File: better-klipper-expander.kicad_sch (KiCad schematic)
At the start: 90 parts, among them J1 24V IN, J10 TH1, J11 VFAN_SEL1, J12 Neopixel, J13 VFAN_SEL2, J2 USB4105-GF-A, J3 FAN0, J4 FAN1, J5 FAN2, J6 TH0, J7 FAN3, J8 FAN4, J9 FAN5, Q1 AO3400C, Q2 AO3400C, Q3 AO3400C, Q4 AO3400C, Q5 AO3400C, Q6 AO3400C, U1 W25Q80DVSNIG, U2 XT1861B332MR-G, U3 TPS5450DDAR, U4 RP2040, U5 TXS0101DBVR, Y1 12MHz

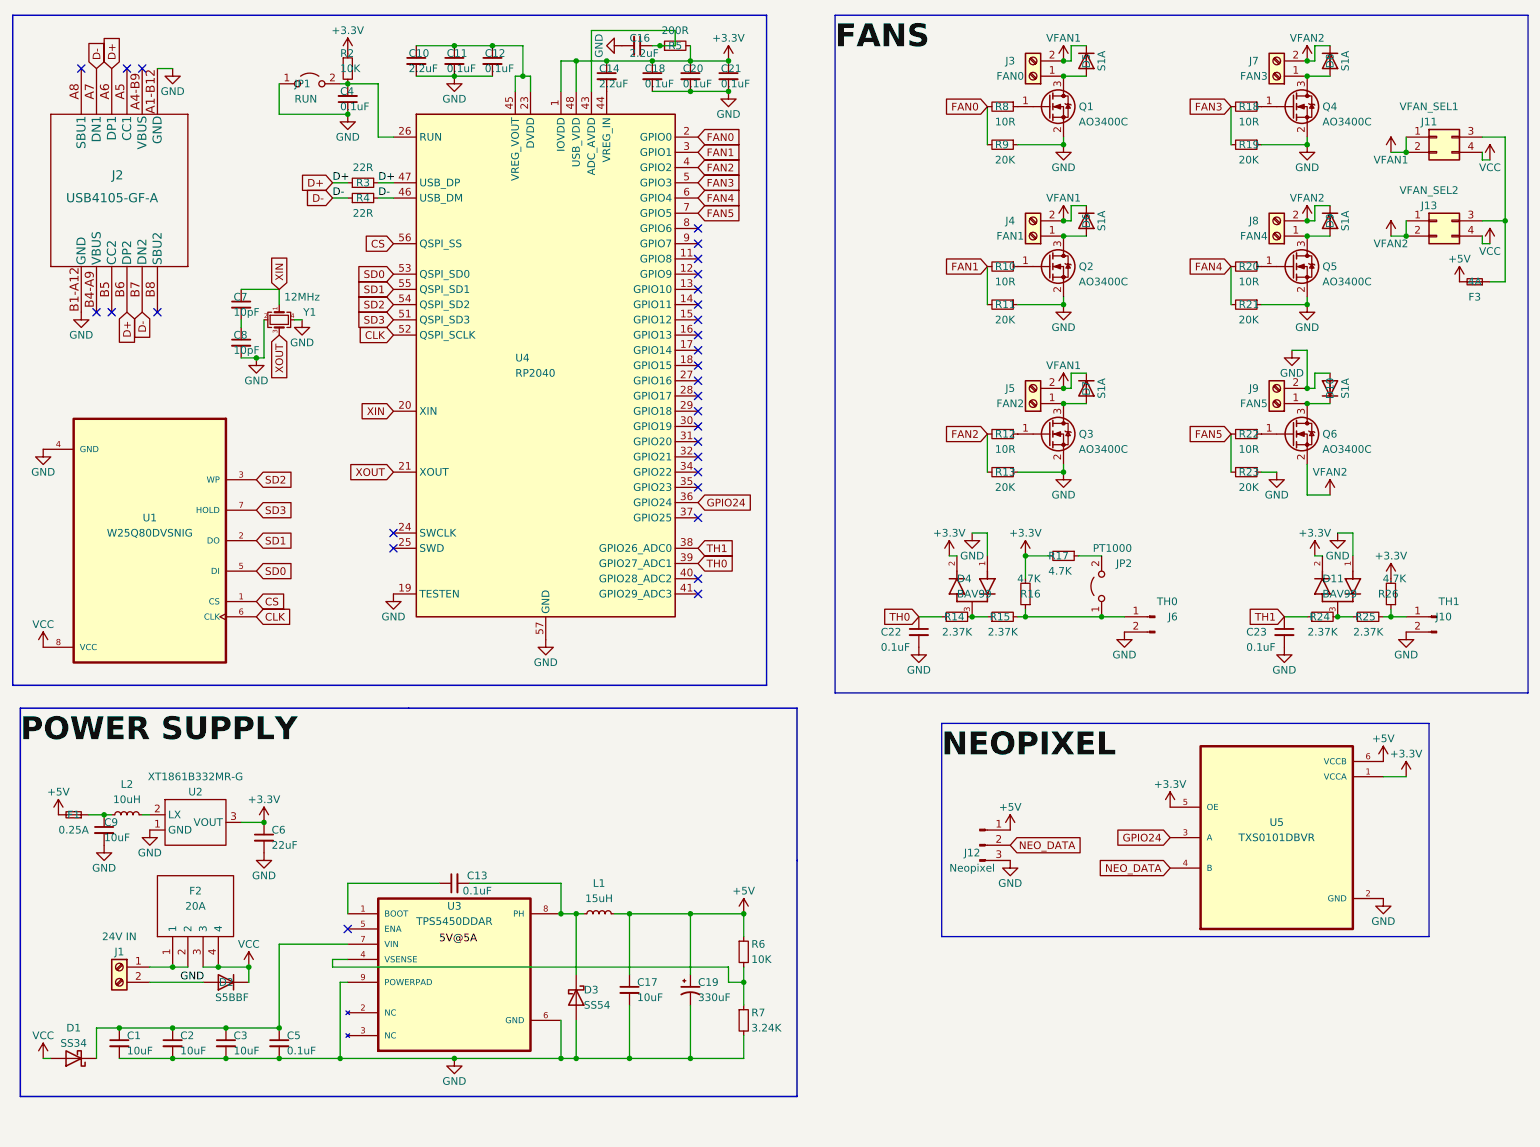
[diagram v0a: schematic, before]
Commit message: Minor updates
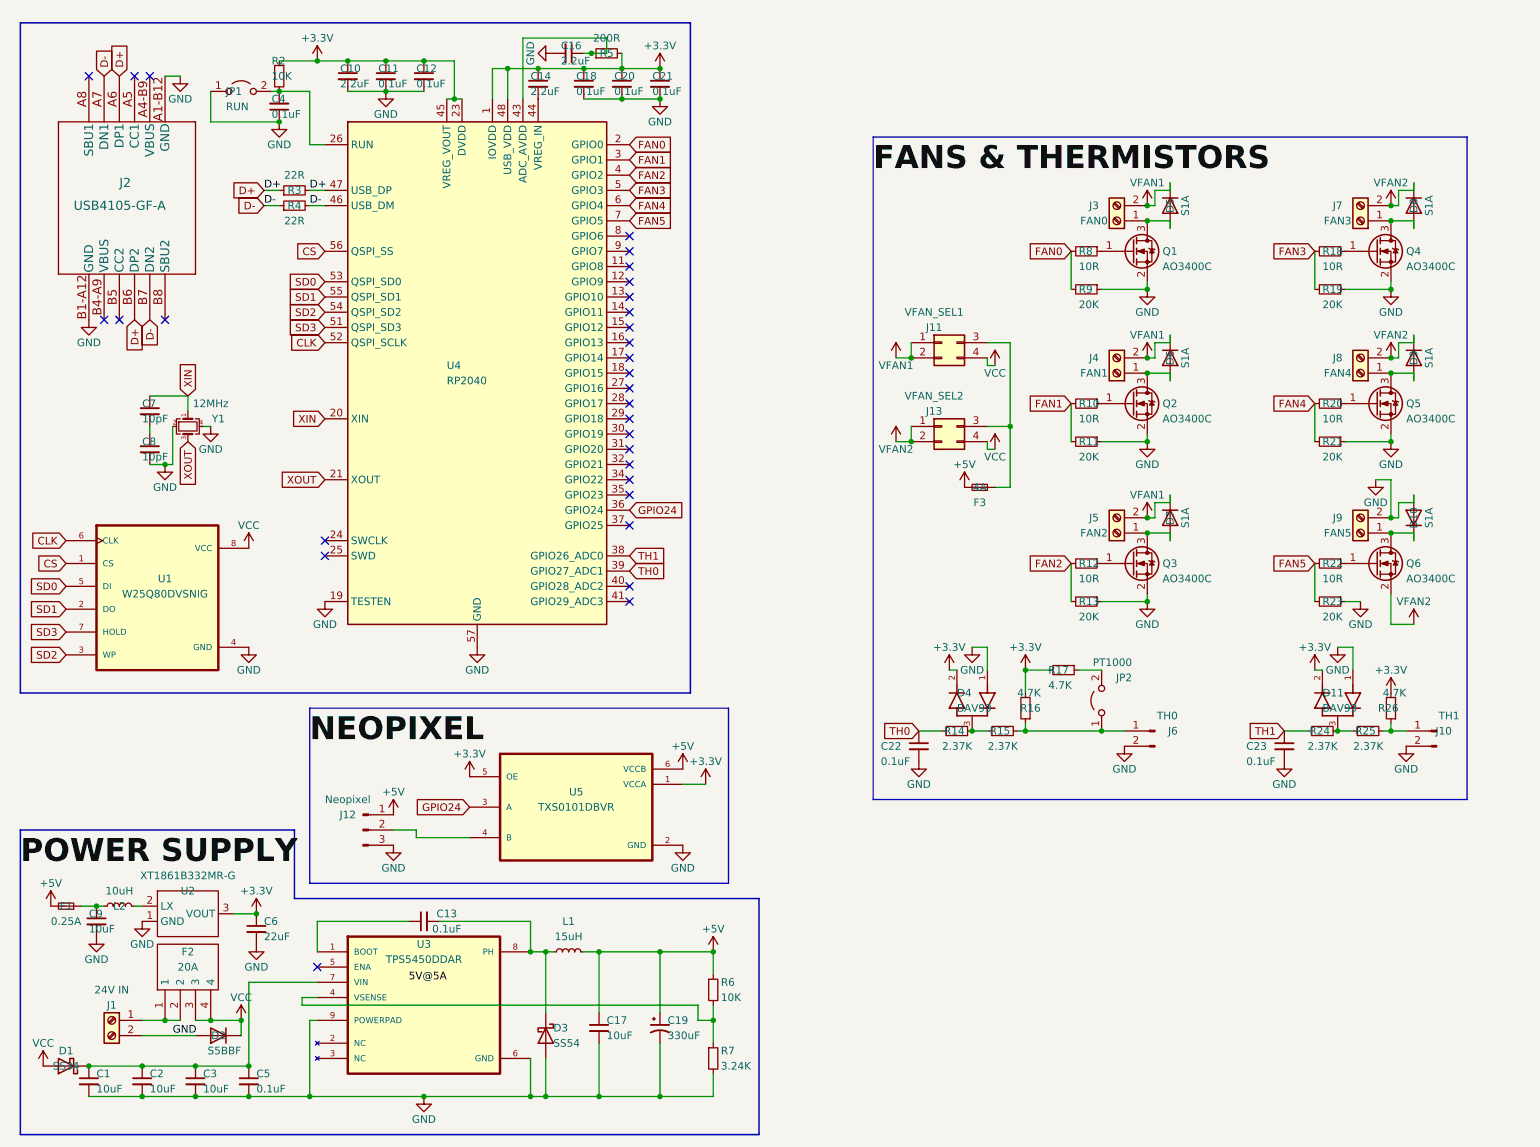
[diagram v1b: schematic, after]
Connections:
- net +3.3V: now also C10.1, C11.1, C12.1, U4.23 (DVDD), U4.45 (VREG_VOUT), U4.50 (DVDD)
- net NEO_DATA: no longer names the net of J12.2 (Pin_2), U5.4 (B)
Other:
- moved on the sheet: C1, C10, C11, C12, C13, C14, C16, C17, C18, C19, C2, C20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
